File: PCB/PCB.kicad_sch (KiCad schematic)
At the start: 5 parts, among them J1 Ultrasonic Sensor, U1 XL1509-3.3, U2 ESP32-C3-DevKitM-1, U3 ESP32-WROOM-32

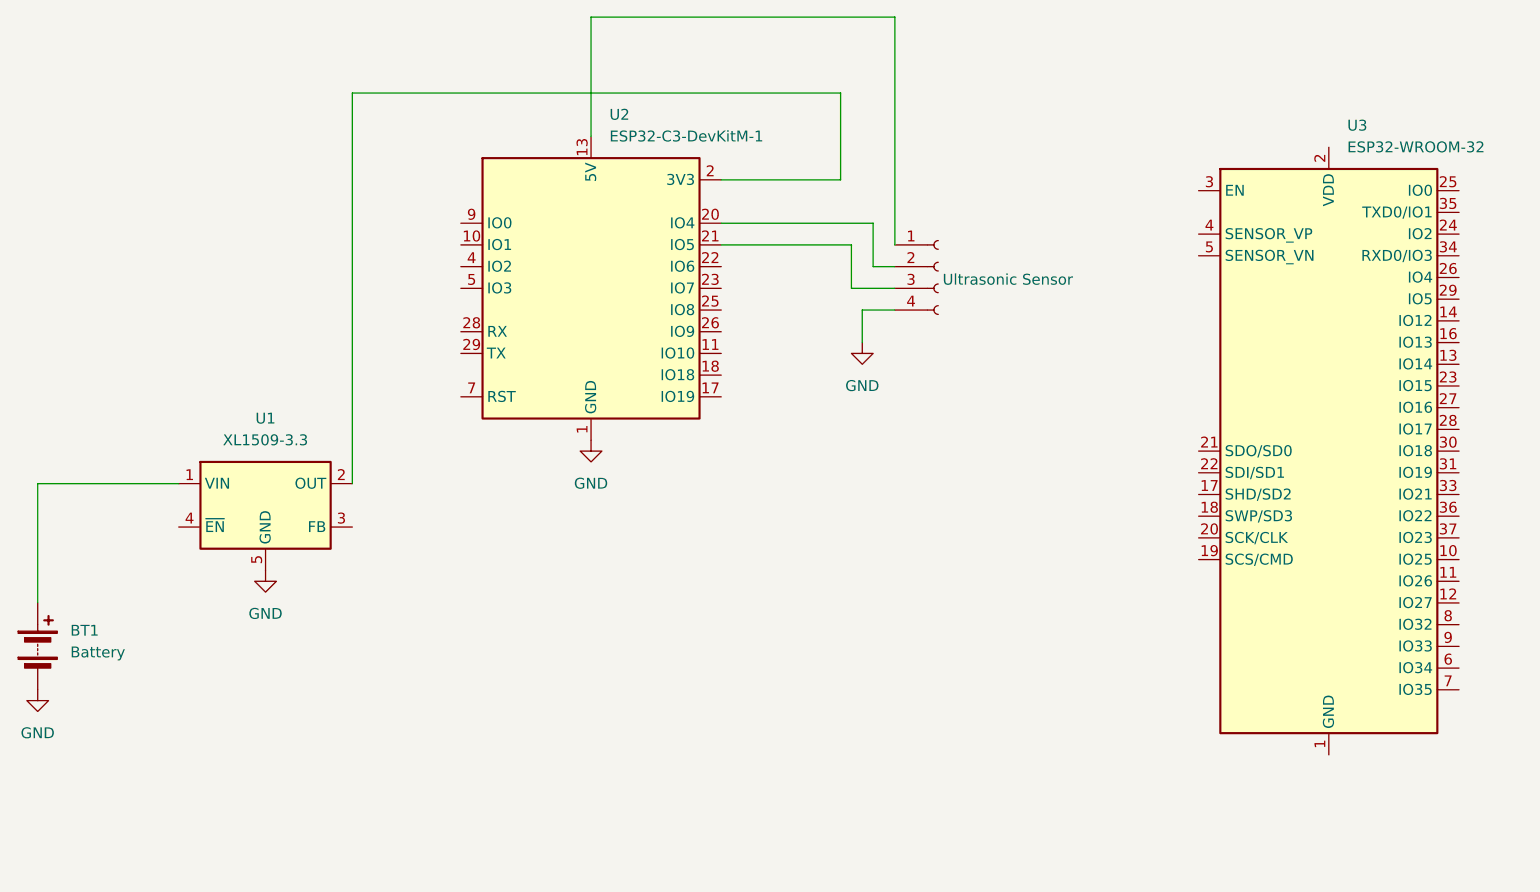
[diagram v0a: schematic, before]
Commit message: updated
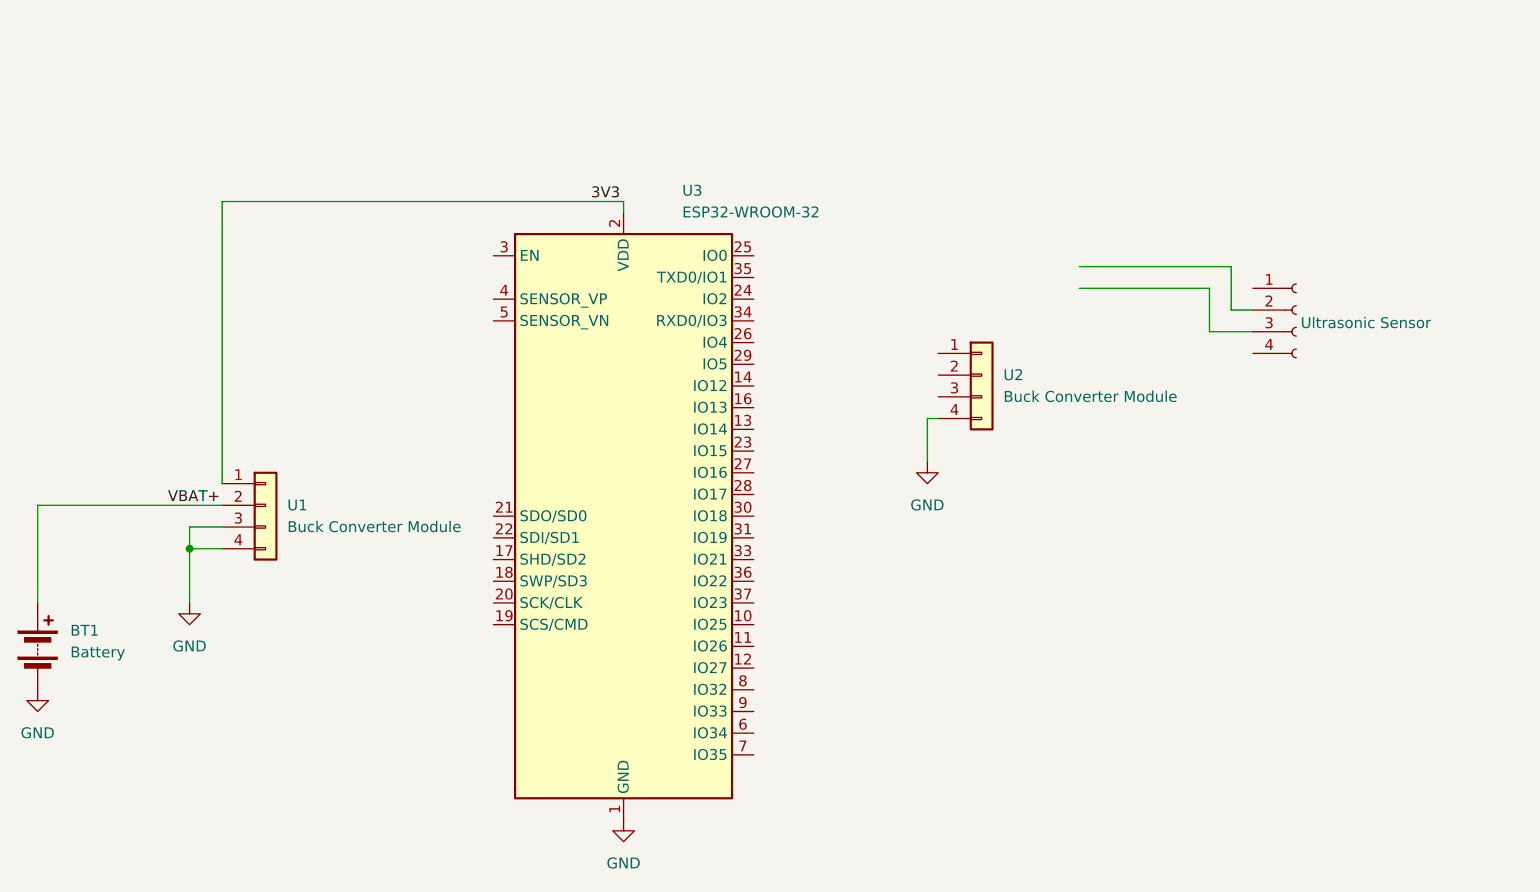
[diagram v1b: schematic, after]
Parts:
- removed U1: XL1509-3.3, Package_SO:SOIC-8_3.9x4.9mm_P1.27mm, symbol Regulator_Switching:XL1509-3.3
- removed U2: ESP32-C3-DevKitM-1, RF_Module:ESP32-C3-DevKitM-1, symbol RF_Module:ESP32-C3-DevKitM-1
- added U1, U2: Buck Converter Module, symbol Connector_Generic:Conn_01x04
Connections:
- net GND: now also U3.1 (GND), U3.15 (GND), U3.38 (GND), U3.39 (GND), U1.3 (Pin_3), U1.4 (Pin_4), U2.4 (Pin_4); no longer J1.4 (Pin_4)
- net 3V3: now reaches U3.2 (VDD)
- net 3V3: now also U1.1 (Pin_1)
- net VBAT+: now reaches BT1.1 (+)
- net VBAT+: now also U1.2 (Pin_2)
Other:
- moved on the sheet: U3
